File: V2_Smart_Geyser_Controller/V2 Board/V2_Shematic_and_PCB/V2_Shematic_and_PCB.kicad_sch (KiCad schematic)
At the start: 1 part, among them J1 1714984

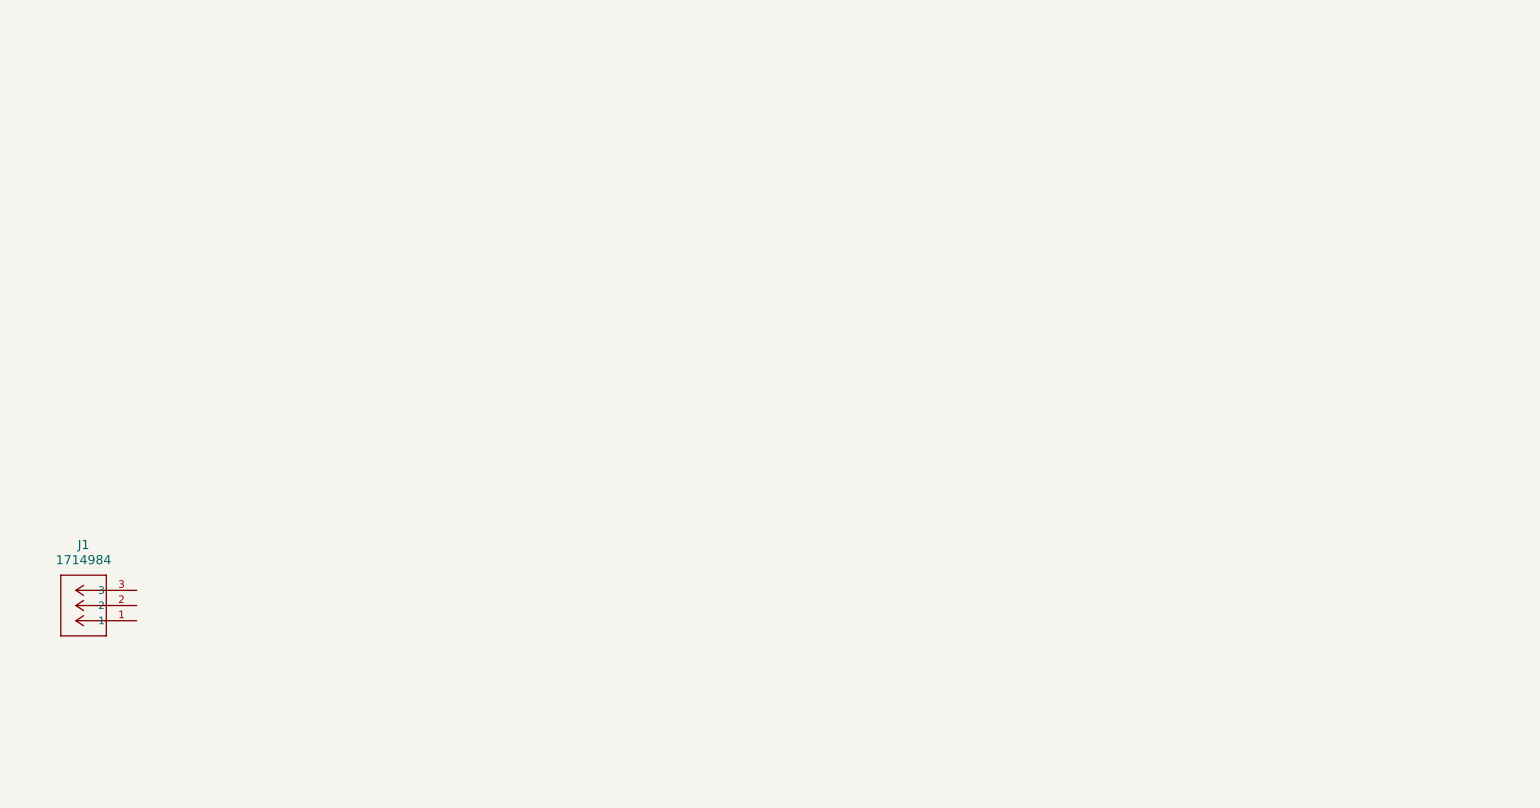
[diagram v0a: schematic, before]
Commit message: Schematic update: AC-DC Converter added. TPS62903RPJR regulator circuit added. The circuit still annotation
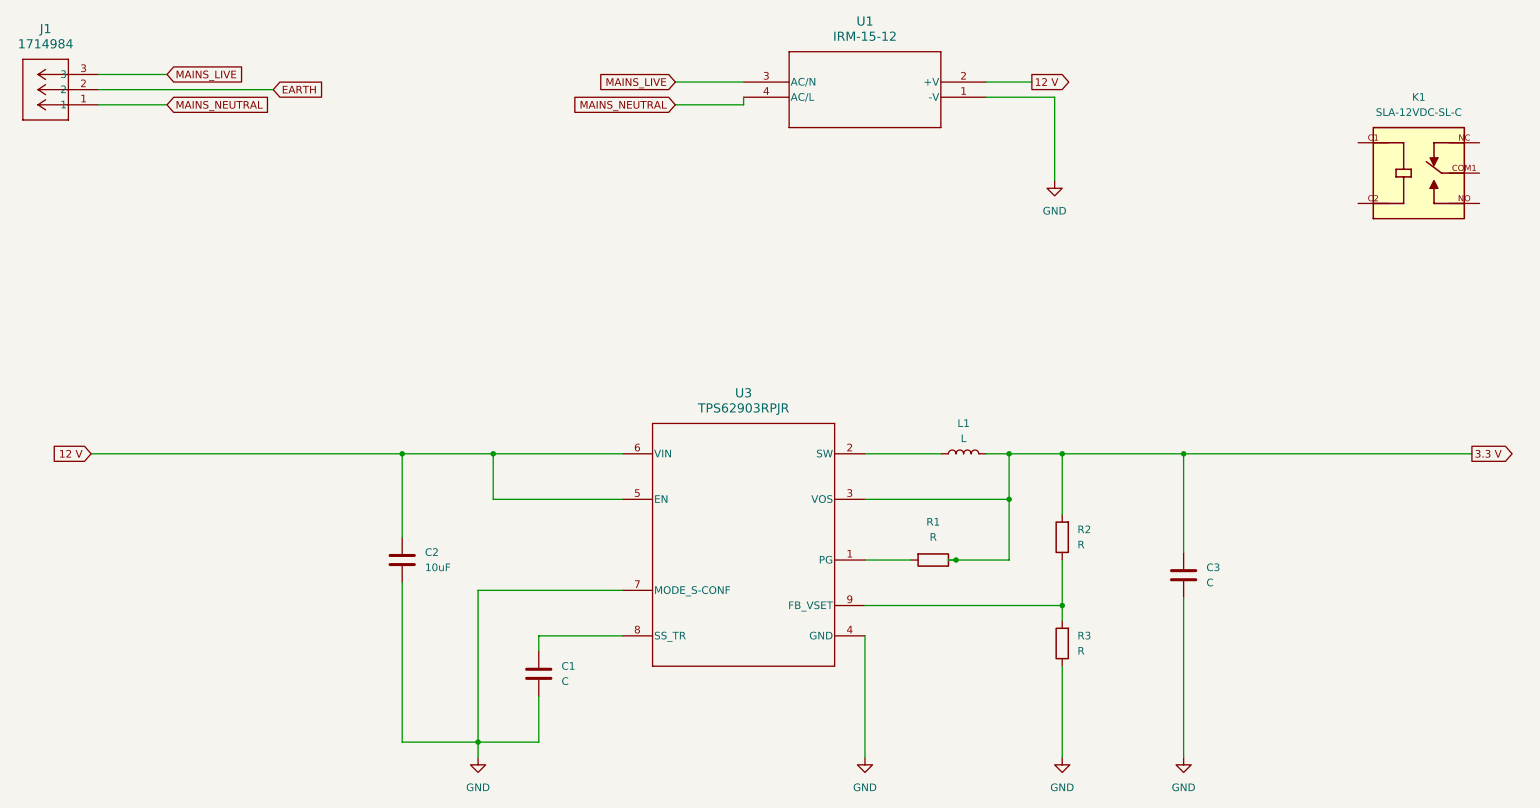
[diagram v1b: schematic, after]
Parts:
- added C1, C3: C, symbol Device:C
- added C2: 10uF, Capacitor_SMD:C_0805_2012Metric, symbol Device:C
- added K1: SLA-12VDC-SL-C, SLA-12VDC-SL-C:RELAY_SLA-12VDC-SL-C, symbol SLA-12VDC-SL-C:SLA-12VDC-SL-C
- added L1: L, symbol Device:L
- added R1, R2, R3: R, symbol Device:R
- added U1: IRM-15-12, footprintsIRM:IRM-15_MWU, symbol 2026-09-15_03-44-23:IRM-15-12
- added U3: TPS62903RPJR, RPJ0009A, symbol 2026-09-19_18-21-30:TPS62903RPJR
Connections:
- net MAINS_NEUTRAL: now reaches J1.1
- net MAINS_NEUTRAL: now also U1.4 (AC/L)
- net EARTH: now reaches J1.2
- net MAINS_LIVE: now reaches J1.3
- net MAINS_LIVE: now also U1.3 (AC/N)
- new net: L1.1, U3.2 (SW)
- new net: R1.2, U3.1 (PG)
- new net: K1.COM1, K1.COM2
- new net: C1.1, U3.8 (SS_TR)
- new net: R2.1, R3.2, U3.9 (FB_VSET)
- new net 12 V: C2.1, U1.2 (+V), U3.5 (EN), U3.6 (VIN)
- new net 3.3 V: C3.1, L1.2, R1.1, R2.2, U3.3 (VOS)
- new net GND: C1.2, C2.2, C3.2, R3.1, U1.1 (-V), U3.4 (GND), U3.7 (MODE_S-CONF)
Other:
- moved on the sheet: J1
